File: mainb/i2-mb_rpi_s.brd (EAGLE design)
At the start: 110 x 106.6 mm, 35 parts, among them IC3 DS1307Z, T1 BC337, T2 BC337, X9 eth (mb->rpi)

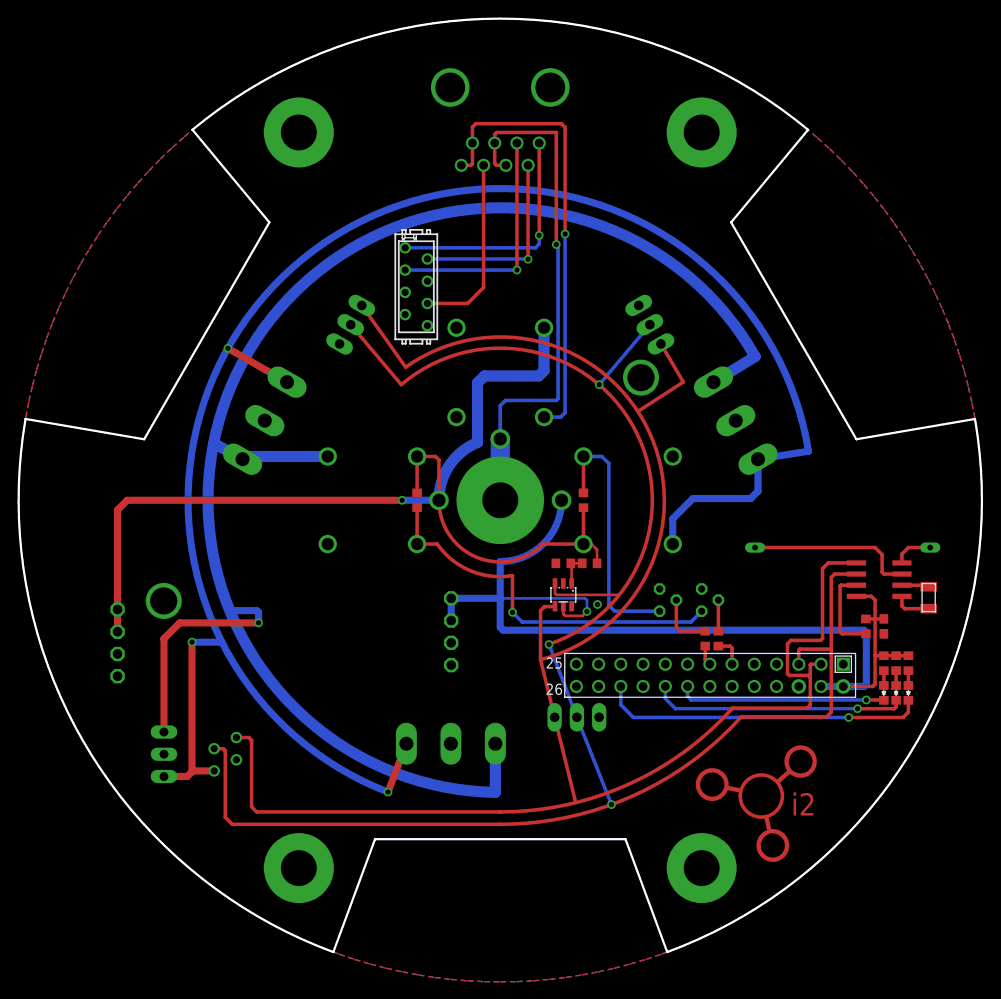
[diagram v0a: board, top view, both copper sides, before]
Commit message: 11.12.13 18:50
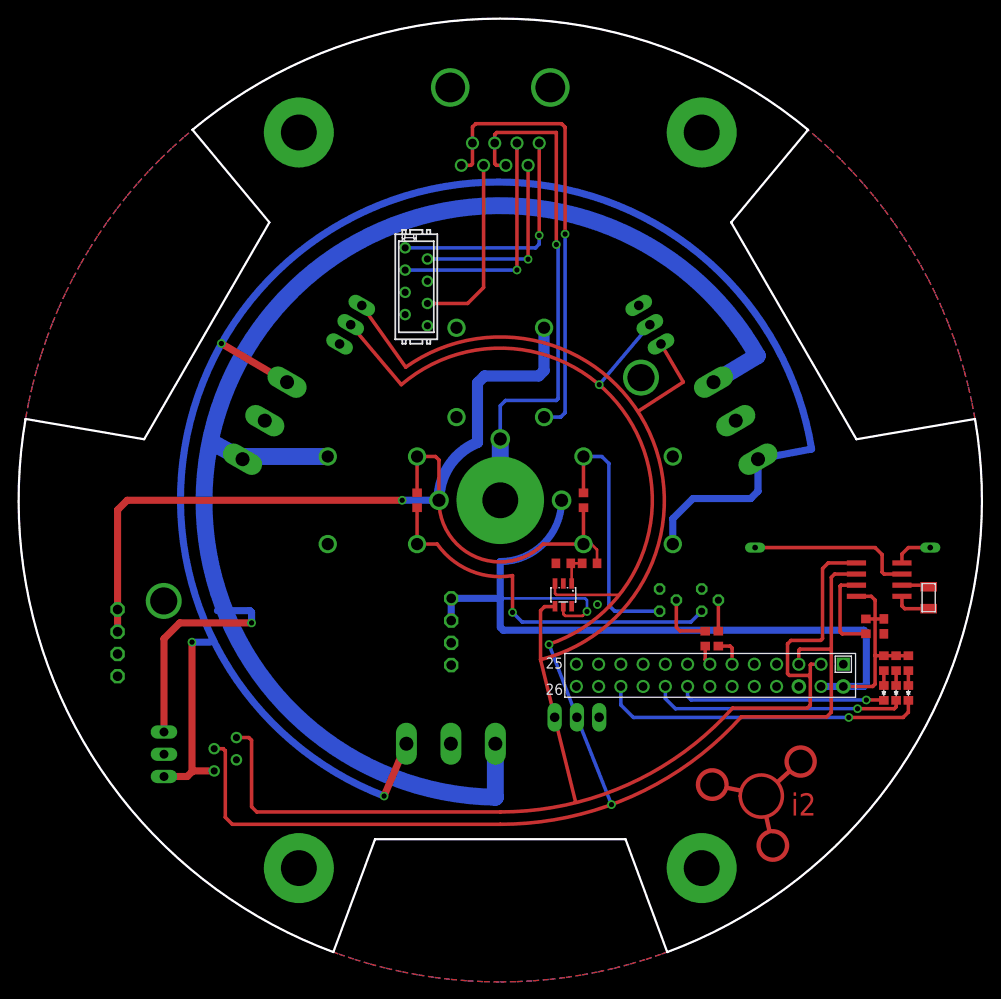
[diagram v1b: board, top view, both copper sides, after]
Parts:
- added U$1: (no value), isfar2-logo:I2-LOGO
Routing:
- net LOGO: track 6.78 -> 0.00 mm
- net +5V: track 123.1 -> 124.7 mm
- net +12V_OUT: track 109.3 -> 110.7 mm
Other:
- board text removed: "i2"
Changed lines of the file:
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@@
 <?xml version="1.0" encoding="utf-8"?>
 <!DOCTYPE eagle SYSTEM "eagle.dtd">
-<eagle version="6.4">
+<eagle version="6.1">
 <drawing>
 <settings>
@@
 <layer number="56" name="wert" color="7" fill="1" visible="no" active="no"/>
 <layer number="57" name="tCAD" color="7" fill="1" visible="no" active="no"/>
+<layer number="58" name="bCAD" color="11" fill="1" visible="no" active="no"/>
 <layer number="91" name="Nets" color="2" fill="1" visible="no" active="no"/>
 <layer number="92" name="Busses" color="1" fill="1" visible="no" active="no"/>
@@
 <wire x1="-19.063" y1="-51.591" x2="-54.210675" y2="9.286115625" width="0.254" layer="20" curve="-79.44085"/>
 <wire x1="-35.147" y1="42.305" x2="35.147" y2="42.305" width="0.254" layer="20" curve="-79.439614"/>
-<text x="33.2" y="-36" size="2.54" layer="1" ratio="20">i2</text>
 </plain>
 <attributes>
@@
 </class>
 </classes>
-<designrules name="default">
+<designrules>
 <description language="de">&lt;b&gt;EAGLE Design Rules&lt;/b&gt;
 &lt;p&gt;
@@
 <attribute name="VALUE" x="-35.21" y="-31.54" size="1.27" layer="28" rot="MR90"/>
 </element>
+<element name="U$1" library="isfar2-logo" package="I2-LOGO" value="" x="30" y="-33.4"/>
 </elements>
 <signals>
-<signal name="SCL">
+<signal name="SCL" airwireshidden="yes">
 <contactref element="IC1" pad="3"/>
 <contactref element="IC3" pad="6"/>
@@
 <wire x1="0" y1="-37" x2="12.7" y2="-34.75" width="0" layer="19" extent="1-1"/>
 </signal>
-<signal name="SDA">
+<signal name="SDA" airwireshidden="yes">
 <contactref element="IC1" pad="4"/>
 <contactref element="IC3" pad="5"/>
@@
 <wire x1="10.4" y1="-5" x2="9.5" y2="-5" width="0.3048" layer="1"/>
 </signal>
-<signal name="+5V">
+<signal name="+5V" airwireshidden="yes">
 <contactref element="U$5" pad="NO"/>
 <contactref element="PWR4" pad="1"/>
@@
 <contactref element="PWR2" pad="1"/>
 <contactref element="PWR1" pad="1"/>
-<wire x1="-10.72" y1="-27.8" x2="-12.82" y2="-33.32" width="0.8128" layer="1"/>
-<wire x1="29.43" y1="4.690590625" x2="35.2" y2="5.6" width="0.8128" layer="16"/>
-<wire x1="-12.82" y1="-33.32" x2="35.2" y2="5.6" width="0.8128" layer="16" curve="-239.803468"/>
-<via x="-12.82" y="-33.32" extent="1-16" drill="0.6"/>
-<wire x1="-24.35" y1="13.48940625" x2="-31.1" y2="17.35" width="0.8128" layer="1"/>
-<via x="-31.1" y="17.35" extent="1-16" drill="0.6"/>
+<wire x1="-10.72" y1="-27.8" x2="-13.27" y2="-33.77" width="0.8128" layer="1"/>
+<wire x1="29.43" y1="4.690590625" x2="35.55" y2="5.85" width="0.8128" layer="16"/>
+<wire x1="-13.27" y1="-33.77" x2="35.55" y2="5.85" width="0.8128" layer="16" curve="-239.803468"/>
+<via x="-13.27" y="-33.77" extent="1-16" drill="0.6"/>
+<wire x1="-24.35" y1="13.48940625" x2="-31.85" y2="17.9" width="0.8128" layer="1"/>
+<via x="-31.85" y="17.9" extent="1-16" drill="0.6"/>
 <wire x1="19.7" y1="-5" x2="19.7" y2="-2.1" width="0.8128" layer="16"/>
 <wire x1="19.7" y1="-2.1" x2="22" y2="0.2" width="0.8128" layer="16"/>
@@
 <wire x1="-35.2" y1="-31" x2="-35.2" y2="-16.2" width="0.8128" layer="1"/>
 <via x="-35.2" y="-16.2" extent="1-16" drill="0.6"/>
-<wire x1="-35.2" y1="-16.2" x2="-31.8" y2="-16.2" width="0.8128" layer="16"/>
+<wire x1="-35.2" y1="-16.2" x2="-33.15" y2="-16.2" width="0.8128" layer="16"/>
 <contactref element="I2C_1" pad="4"/>
 <wire x1="-32.67" y1="-30.905" x2="-35.105" y2="-30.905" width="0.8128" layer="1"/>
 <wire x1="-35.105" y1="-30.905" x2="-35.2" y2="-31" width="0.4064" layer="1"/>
-<wire x1="-12.82" y1="-33.32" x2="-32.67" y2="-30.905" width="0" layer="19" extent="1-1"/>
-<wire x1="-24.35" y1="13.48940625" x2="-31.8" y2="-16.2" width="0" layer="19" extent="16-16"/>
+<wire x1="-13.27" y1="-33.77" x2="-32.67" y2="-30.905" width="0" layer="19" extent="1-1"/>
+<wire x1="-24.35" y1="13.48940625" x2="-33.15" y2="-16.2" width="0" layer="19" extent="16-16"/>
 </signal>
 <signal name="GND">
@@
 <contactref element="X_ETH" pad="5"/>
 <via x="0" y="0" extent="1-16" drill="4.1" diameter="10"/>
-<wire x1="0" y1="0" x2="0" y2="7" width="2.1844" layer="16"/>
+<wire x1="0" y1="0" x2="0" y2="7" width="1.9304" layer="16"/>
 <wire x1="0" y1="7" x2="0" y2="10.8" width="0.4064" layer="16"/>
 <wire x1="0" y1="10.8" x2="0.6" y2="11.4" width="0.4064" layer="16"/>
@@
 <wire x1="23.92" y1="-18.72" x2="23.4" y2="-18.2" width="0.4064" layer="1"/>
 </signal>
-<signal name="+12V_OUT">
+<signal name="+12V_OUT" airwireshidden="yes">
 <contactref element="U$7" pad="NO"/>
 <contactref element="PWR4" pad="3"/>
@@
 <contactref element="PWR1" pad="3"/>
 <contactref element="PWR3" pad="3"/>
-<wire x1="-29.430003125" y1="4.690590625" x2="-32.7" y2="6.5" width="1.27" layer="16"/>
-<wire x1="-0.56" y1="-27.8" x2="-0.56" y2="-33.36" width="1.27" layer="16"/>
-<wire x1="24.350003125" y1="13.48940625" x2="29.1" y2="16.4" width="1.27" layer="16"/>
-<wire x1="-0.56" y1="-33.36" x2="29.1" y2="16.4" width="1.27" layer="16" curve="-239.633819"/>
-<wire x1="-19.7" y1="5" x2="-29.12059375" y2="5" width="1.27" layer="16"/>
+<wire x1="-29.430003125" y1="4.690590625" x2="-32.7" y2="6.5" width="1.9304" layer="16"/>
+<wire x1="-0.56" y1="-27.8" x2="-0.56" y2="-33.91" width="1.9304" layer="16"/>
+<wire x1="24.350003125" y1="13.48940625" x2="29.35" y2="16.5" width="1.9304" layer="16"/>
+<wire x1="-0.56" y1="-33.91" x2="29.35" y2="16.5" width="1.9304" layer="16" curve="-239.633819"/>
+<wire x1="-19.7" y1="5" x2="-29.12059375" y2="5" width="1.9304" layer="16"/>
 <wire x1="-29.12059375" y1="5" x2="-29.430003125" y2="4.690590625" width="1.27" layer="16"/>
 <wire x1="-38.4" y1="-26.46" x2="-38.4" y2="-15.8" width="0.8128" layer="1"/>
 <wire x1="-38.4" y1="-15.8" x2="-36.6" y2="-14" width="0.8128" layer="1"/>
-<wire x1="-36.6" y1="-14" x2="-27.6" y2="-14" width="0.8128" layer="1"/>
-<via x="-27.6" y="-14" extent="1-16" drill="0.6"/>
-<wire x1="-27.6" y1="-14" x2="-27.6" y2="-12.8" width="0.8128" layer="16"/>
-<wire x1="-27.6" y1="-12.8" x2="-27.8" y2="-12.6" width="0.8128" layer="16"/>
-<wire x1="-27.8" y1="-12.6" x2="-30.8" y2="-12.6" width="0.8128" layer="16"/>
-<wire x1="-29.430003125" y1="4.690590625" x2="-30.8" y2="-12.6" width="0" layer="19" extent="16-16"/>
-<wire x1="-0.56" y1="-27.8" x2="-27.6" y2="-14" width="0" layer="19" extent="1-1"/>
+<wire x1="-36.6" y1="-14" x2="-28.4" y2="-14" width="0.8128" layer="1"/>
+<via x="-28.4" y="-14" extent="1-16" drill="0.6"/>
+<wire x1="-28.4" y1="-14" x2="-28.4" y2="-12.8" width="0.8128" layer="16"/>
+<wire x1="-28.4" y1="-12.8" x2="-28.6" y2="-12.6" width="0.8128" layer="16"/>
+<wire x1="-28.6" y1="-12.6" x2="-32.3" y2="-12.6" width="0.8128" layer="16"/>
+<wire x1="-29.430003125" y1="4.690590625" x2="-28.6" y2="-12.6" width="0" layer="19" extent="16-16"/>
+<wire x1="-0.56" y1="-27.8" x2="-28.4" y2="-14" width="0" layer="19" extent="1-1"/>
 </signal>
 <signal name="LED2">
@@
 <wire x1="46.6" y1="-24.2" x2="46" y2="-24.8" width="0.4064" layer="1"/>
 </signal>
-<signal name="LOGO" airwireshidden="yes">
-<wire x1="30.40555625" y1="-36.284284375" x2="30.752065625" y2="-37.817265625" width="0.5" layer="1"/>
-<wire x1="30.492371875" y1="-37.922428125" x2="31.04254375" y2="-37.796675" width="0.5" layer="1" curve="340"/>
-<wire x1="31.73215" y1="-32.11245" x2="33.078153125" y2="-30.904828125" width="0.5" layer="1"/>
-<wire x1="33.29179375" y1="-31.08246875" x2="32.92600625" y2="-30.662234375" width="0.5" layer="1" curve="340"/>
-<wire x1="25.833675" y1="-32.519990625" x2="25.7159375" y2="-33.07365" width="0.5" layer="1" curve="340"/>
-<wire x1="27.4" y1="-33.75" x2="27.4" y2="-33.8" width="0.4064" layer="1" curve="-358.81"/>
-<wire x1="27.425503125" y1="-33.141871875" x2="25.79104375" y2="-32.81219375" width="0.5" layer="1"/>
-<wire x1="27.425503125" y1="-33.141871875" x2="27.4" y2="-33.75" width="0" layer="19" extent="1-1"/>
-<wire x1="25.7159375" y1="-33.07365" x2="25.79104375" y2="-32.81219375" width="0" layer="19" extent="1-1"/>
-<wire x1="30.40555625" y1="-36.284284375" x2="27.4" y2="-33.8" width="0" layer="19" extent="1-1"/>
-<wire x1="30.492371875" y1="-37.922428125" x2="30.752065625" y2="-37.817265625" width="0" layer="19" extent="1-1"/>
-<wire x1="31.73215" y1="-32.11245" x2="30.40555625" y2="-36.284284375" width="0" layer="19" extent="1-1"/>
-<wire x1="33.29179375" y1="-31.08246875" x2="33.078153125" y2="-30.904828125" width="0" layer="19" extent="1-1"/>
-</signal>
 </signals>
